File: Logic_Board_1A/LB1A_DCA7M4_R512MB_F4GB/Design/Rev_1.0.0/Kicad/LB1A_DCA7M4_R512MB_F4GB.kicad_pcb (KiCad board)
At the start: 6 copper layers, 50 x 50 mm, 143 parts, among them U1 STM32MP157CAC3, U2 AS4C256M16D3LC-12BCN, U3 S40FC004C1B2C00000, U4 STPMIC1BPQR, U5 DF40C-70DP-0.4V(51), U6 DF40C-70DP-0.4V(51), U7 DF40C-70DP-0.4V(51), X1 32.768kHz, X2 24MHz

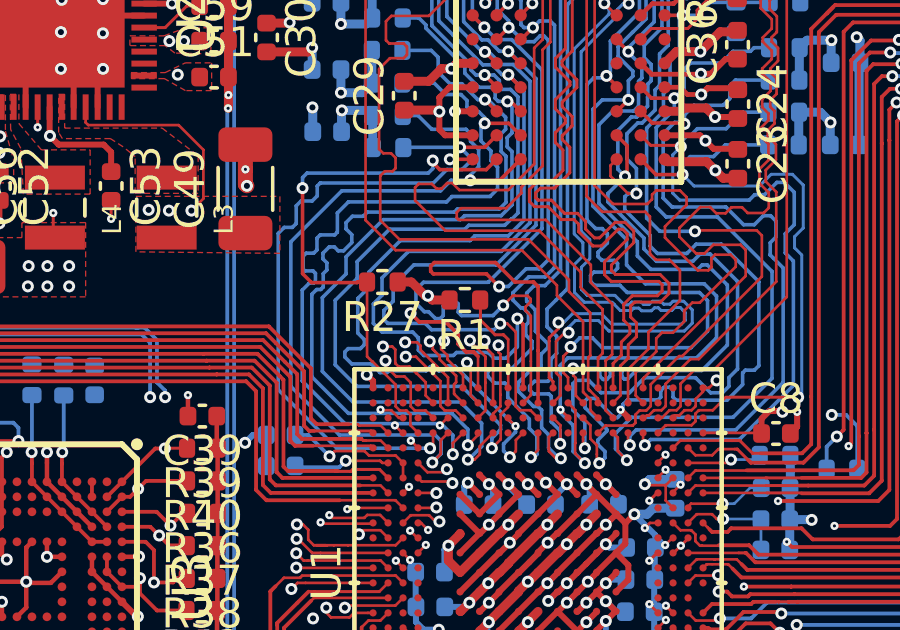
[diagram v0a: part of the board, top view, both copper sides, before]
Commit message: Improvements to PCB
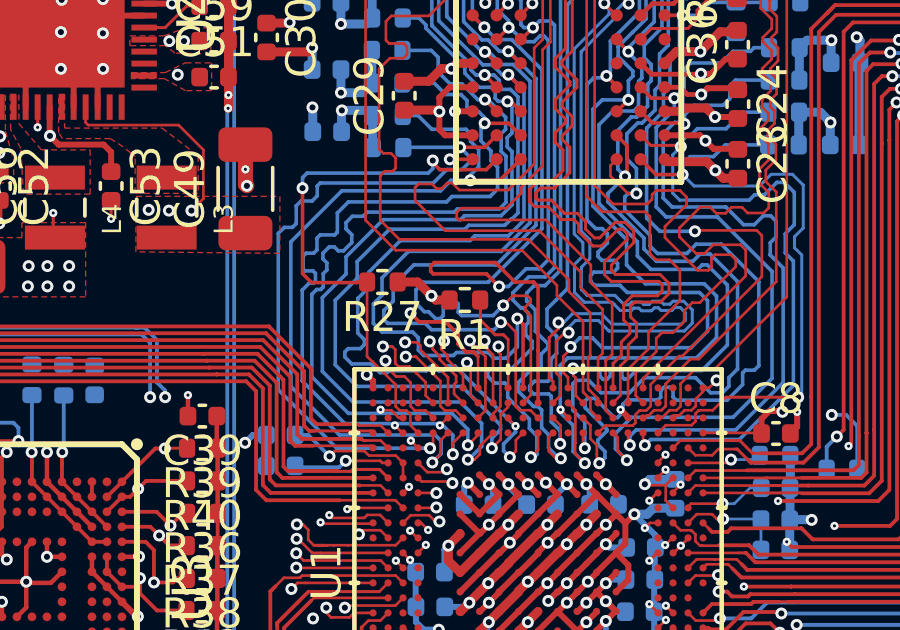
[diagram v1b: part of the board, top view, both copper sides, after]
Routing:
- net DDR_DQ3: track 24.7 -> 35.3 mm
- net DDR_DQ5: track 26.2 -> 34.4 mm
- net DDR_DQ0: track 25.1 -> 32.2 mm
- net DDR_DQS0_N: track 26.5 -> 33.5 mm
- net DDR_DQ4: track 27.3 -> 34.1 mm
- net DDR_DQ1: track 25.3 -> 31.6 mm
- net DDR_DQM0: track 25.6 -> 31.6 mm
- net DDR_DQ2: track 26.1 -> 31.6 mm
- net DDR_DQ7: track 26.9 -> 32.1 mm
- net DDR_DQ6: track 27.2 -> 32.2 mm
- net DDR_DQS0_P: track 27.1 -> 31.6 mm
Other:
- net class DDR_DiffPairs: clearance 0.1016 -> 0.0762
- net class Default: clearance 0.1016 -> 0.0762
- net class Gnd_Lines: clearance 0.1016 -> 0.0762
- rule trace_clearance: 0.1016 -> 0.0762

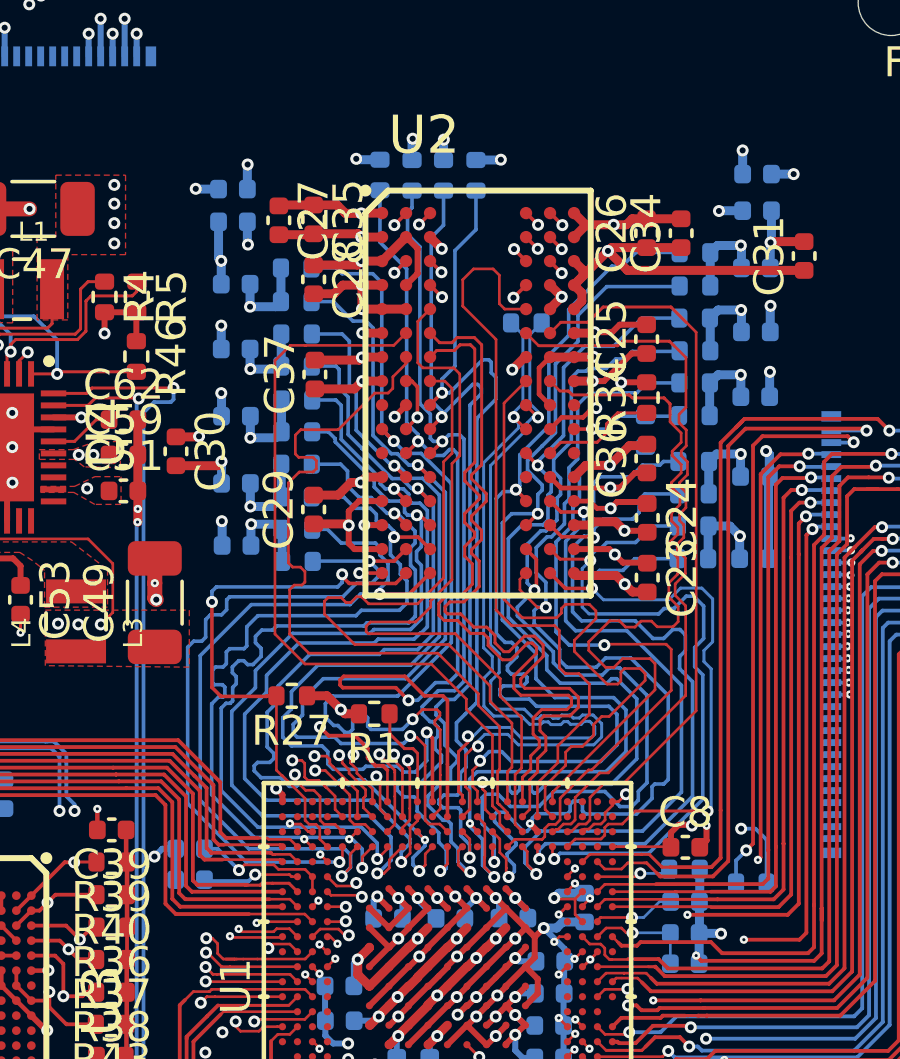
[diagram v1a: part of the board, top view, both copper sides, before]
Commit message: pcb improvements
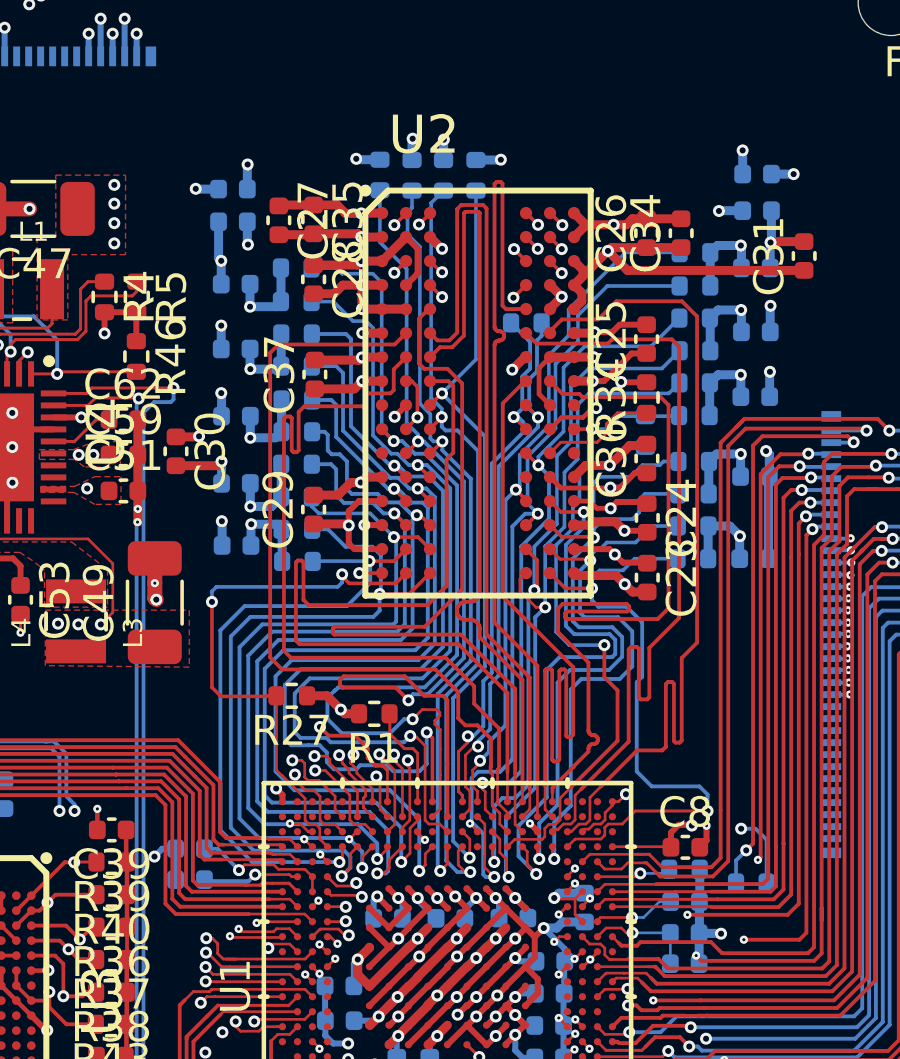
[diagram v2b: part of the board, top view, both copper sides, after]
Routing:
- net DDR_A14: track 34.8 -> 24.0 mm
- net DDR_A12: track 32.7 -> 22.9 mm
- net DDR_A11: track 32.9 -> 23.4 mm
- net DDR_A10: track 30.4 -> 22.2 mm
- net DDR_CLK_P: track 26.7 -> 18.8 mm
- net DDR_CLK_N: track 25.8 -> 18.4 mm
- net DDR_A1: track 35.1 -> 28.2 mm
- net DDR_A6: track 24.1 -> 18.7 mm
- net DDR_DQ13: track 23.1 -> 28.3 mm
- net DDR_DQ15: track 24.6 -> 29.7 mm
- net DDR_A4: track 25.1 -> 20.2 mm
- net DDR_DQ14: track 22.8 -> 27.3 mm
- net DDR_RASN: track 29.5 -> 25.5 mm
- net DDR_CASN: track 30.0 -> 26.6 mm
- net DDR_WEN: track 29.2 -> 25.9 mm
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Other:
- net class DDR_DiffPairs: clearance 0.0762 -> 0.1016
- net class Default: clearance 0.0762 -> 0.1016
- net class Gnd_Lines: clearance 0.0762 -> 0.1016
- rule trace_clearance: 0.0762 -> 0.1016
